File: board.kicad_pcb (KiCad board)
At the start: 4 copper layers, 55 x 52 mm, 66 parts, among them J1 PROVISIONAL_PS1_BARE_MALE_PIN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, J2 USB-C USB2 HRO TYPE-C-31-M-12, Q1 2N7002 DATA OD, Q2 2N7002 ACK OD, Q3 MMBT3904 AUTO-BOOT, Q4 MMBT3904 AUTO-RESET, SW1 RESET K2-1107ST-A4SW-06, SW2 BOOT K2-1107ST-A4SW-06, U1 ESP32-WROOM-32, U2 AP63203WU-7 3.3V 2A PS1 BUCK, U3 AP2112K-3.3 USB LDO, U4 TPS2113APW POWER MUX, U5 CH340C USB-UART, U6 USBLC6-2SC6 ESD

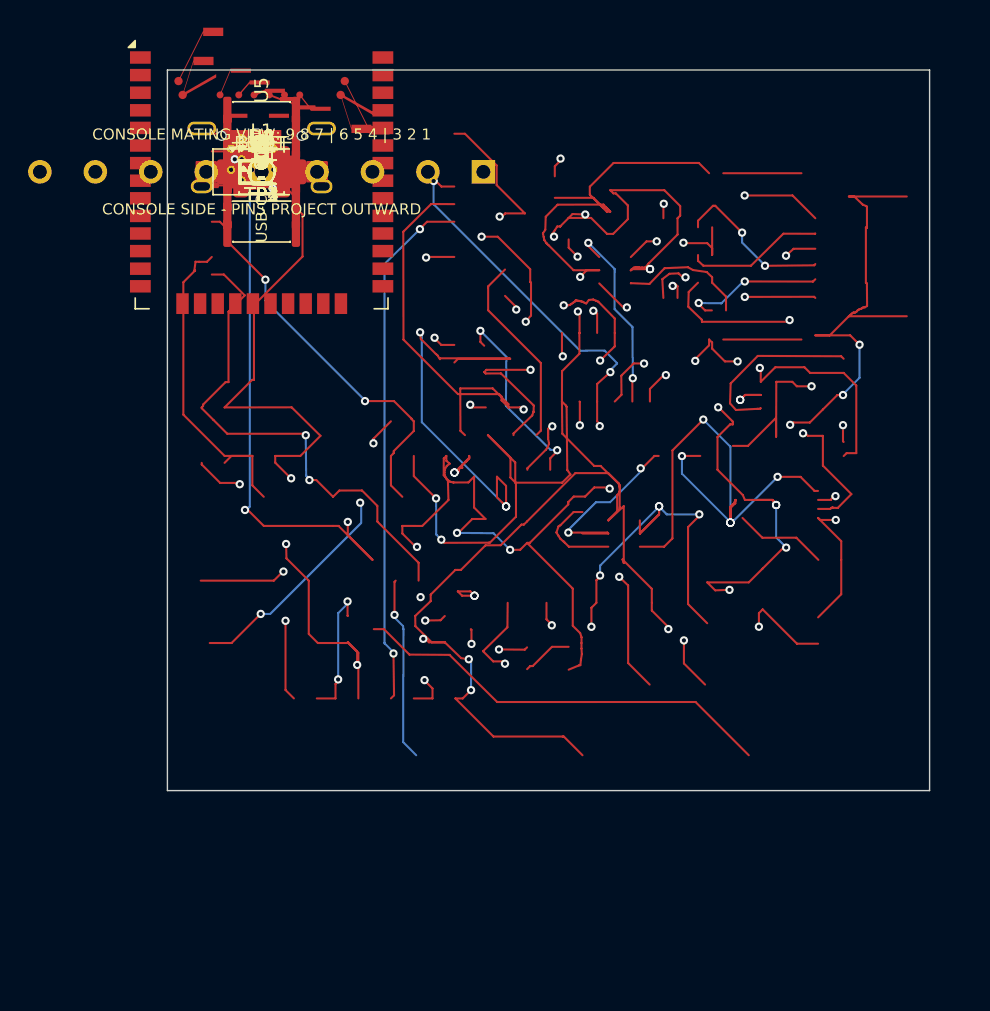
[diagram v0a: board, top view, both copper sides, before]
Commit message: Add V2 modular donor harness board checkpoint
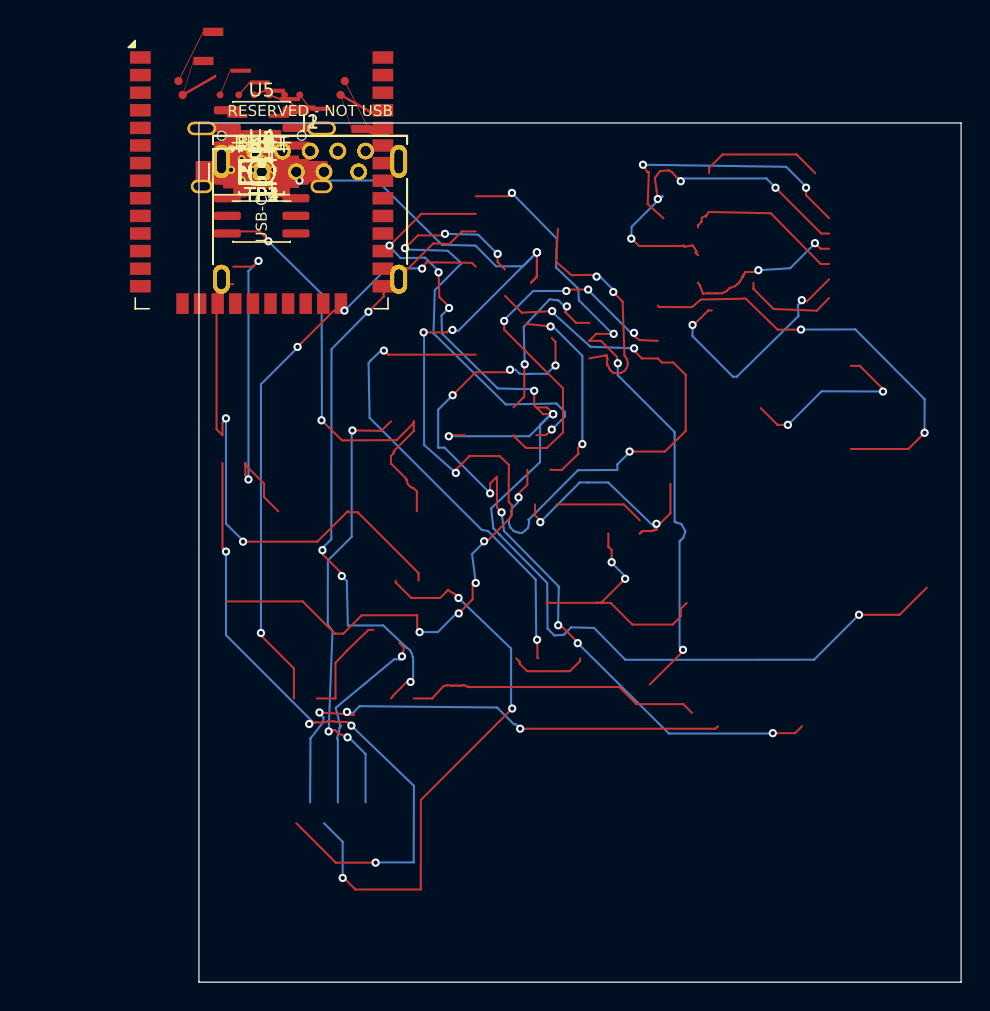
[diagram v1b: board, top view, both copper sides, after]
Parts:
- added J3: USB-C USB2 HRO TYPE-C-31-M-12 PROGRAMMING, PlayBridge:USB_C_Receptacle_HRO_TYPE-C-31-M-12_INTERIOR_FANOUT_V16_C165948_MODEL, F.Cu at (0.00, 0.00)
- J1: value PROVISIONAL_PS1_BARE_MALE_PIN_ARRAY MECHANICAL_TBD NOT_FOR_PRODUCTION -> PS1 DONOR HARNESS / NOT USB; footprint PlayBridge:PROVISIONAL_PS1_MALE_PIN_ARRAY_P4.00_SQ0.64_P16.00_MECH_TBD_3D -> PlayBridge:USB3_A_Molex_48393-0003_AUTHORIZED_COPY
- J2: value USB-C USB2 HRO TYPE-C-31-M-12 -> RESERVED REAR SERIAL / NOT USB / ALL CONTACTS NC; footprint PlayBridge:USB_C_Receptacle_HRO_TYPE-C-31-M-12_INTERIOR_FANOUT_V16_C165948_MODEL -> PlayBridge:USB3_A_Molex_48393-0003_RESERVED_NOT_USB_V2
- U4: footprint PlayBridge:TSSOP-8_3x3mm_P0.65mm_U4_ESCAPE_V2 -> PlayBridge:TSSOP-8_3x3mm_P0.65mm_AUTHORIZED_KICAD_COPY
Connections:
- D3 pad 1: 3V3 -> PS_3V3
- D4 pad 1: 3V3 -> PS_3V3
- D5 pad 1: 3V3 -> PS_3V3
- J1 pad 1: PS_DATA -> (no net)
- J1 pad 3: PS_8V_RAW -> PS_CLK
- J1 pad 5: (no net) -> PS_ATT
- J1 pad 6: PS_ATT -> PS_DATA
- J1 pad 7: PS_CLK -> PS_ACK
- J1 pad 8: (no net) -> PS_8V_RAW
- J1 pad 9: PS_ACK -> (no net)
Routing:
- net GND: track 320.8 -> 0.00 mm, vias 28 -> 0
- net 3V3: track 110.4 -> 0.00 mm, vias 8 -> 0
- net USB_5V: track 62.4 -> 0.00 mm, vias 4 -> 0
- net PS_3V3: track 57.9 -> 0.00 mm, vias 8 -> 0
- net UART_RX: track 56.3 -> 88.4 mm, vias 2 -> 8
- net PS_CLK: track 13.4 -> 41.6 mm, vias 1 -> 3
- net USB_3V3: track 25.3 -> 0.00 mm, vias 2 -> 0
- net AUTO_RESET: track 14.2 -> 34.4 mm, vias 0 -> 4
- net PS_ACK: track 18.0 -> 37.6 mm, vias 1 -> 3
- net PS_8V_RAW: track 18.6 -> 0.00 mm, vias 1 -> 0
- net USB_DTR: track 23.0 -> 40.7 mm
- net USB_DP_B: track 9.98 -> 27.0 mm, vias 0 -> 4
- net PS_DATA: track 30.8 -> 14.4 mm, vias 0 -> 1
- net PS_8V: track 33.4 -> 18.3 mm, vias 6 -> 2
- net USB_DP: track 14.1 -> 0.00 mm, vias 2 -> 0
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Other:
- board size 55 x 52 mm -> 55 x 62 mm
- copper layers 4 -> 2
